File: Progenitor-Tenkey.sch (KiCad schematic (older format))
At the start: 208 parts, among them SW1 SW_Push, U1 ATmega32U4-AU, Y1 16MHz

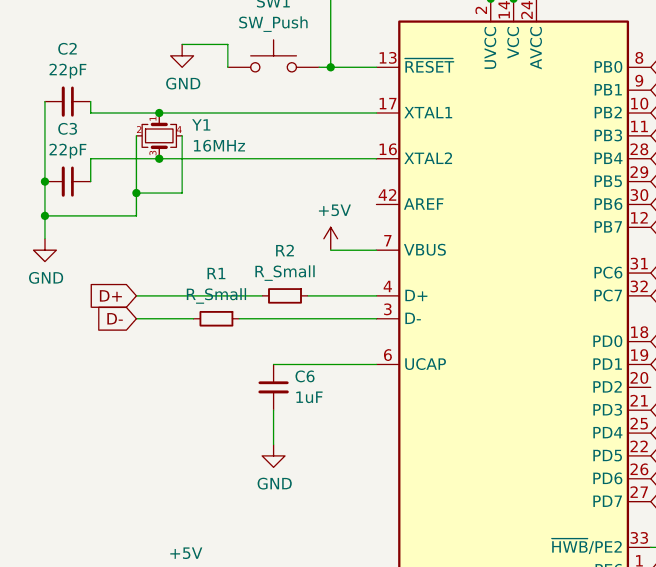
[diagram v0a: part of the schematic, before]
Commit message: More tweaks, regenerated Gerber
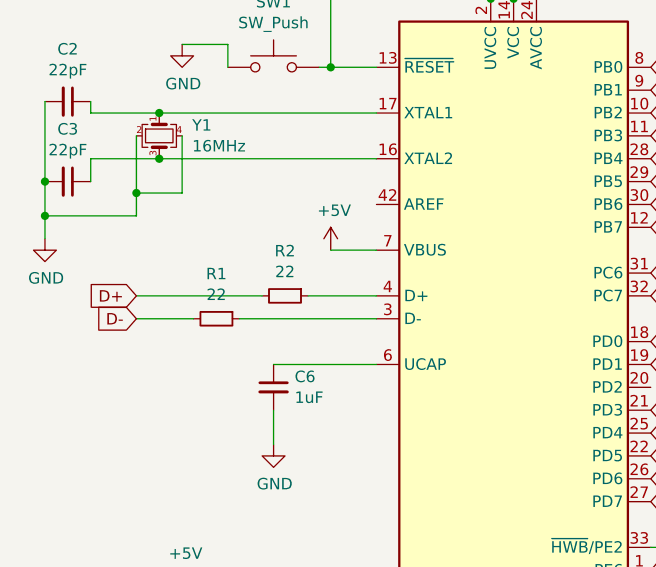
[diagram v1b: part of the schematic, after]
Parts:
- R1, R2: value R_Small -> 22
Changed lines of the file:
@@
 P 1650 2400
 F 0 "R2" V 1454 2400 50  0000 C CNN
-F 1 "R_Small" V 1545 2400 50  0000 C CNN
+F 1 "22" V 1545 2400 50  0000 C CNN
 F 2 "Resistor_SMD:R_0805_2012Metric" H 1650 2400 50  0001 C CNN
 F 3 "~" H 1650 2400 50  0001 C CNN
@@
 P 1350 2500
 F 0 "R1" V 1154 2500 50  0000 C CNN
-F 1 "R_Small" V 1245 2500 50  0000 C CNN
+F 1 "22" V 1245 2500 50  0000 C CNN
 F 2 "Resistor_SMD:R_0805_2012Metric" H 1350 2500 50  0001 C CNN
 F 3 "~" H 1350 2500 50  0001 C CNN
